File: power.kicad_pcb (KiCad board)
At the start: 2 copper layers, 19.6 x 14.7 mm, 13 parts, among them J6 Conn_01x02, J7 Conn_01x05, Q2 FDC6420C, U5 SGM2036_UTDFN, U7 SGM40561

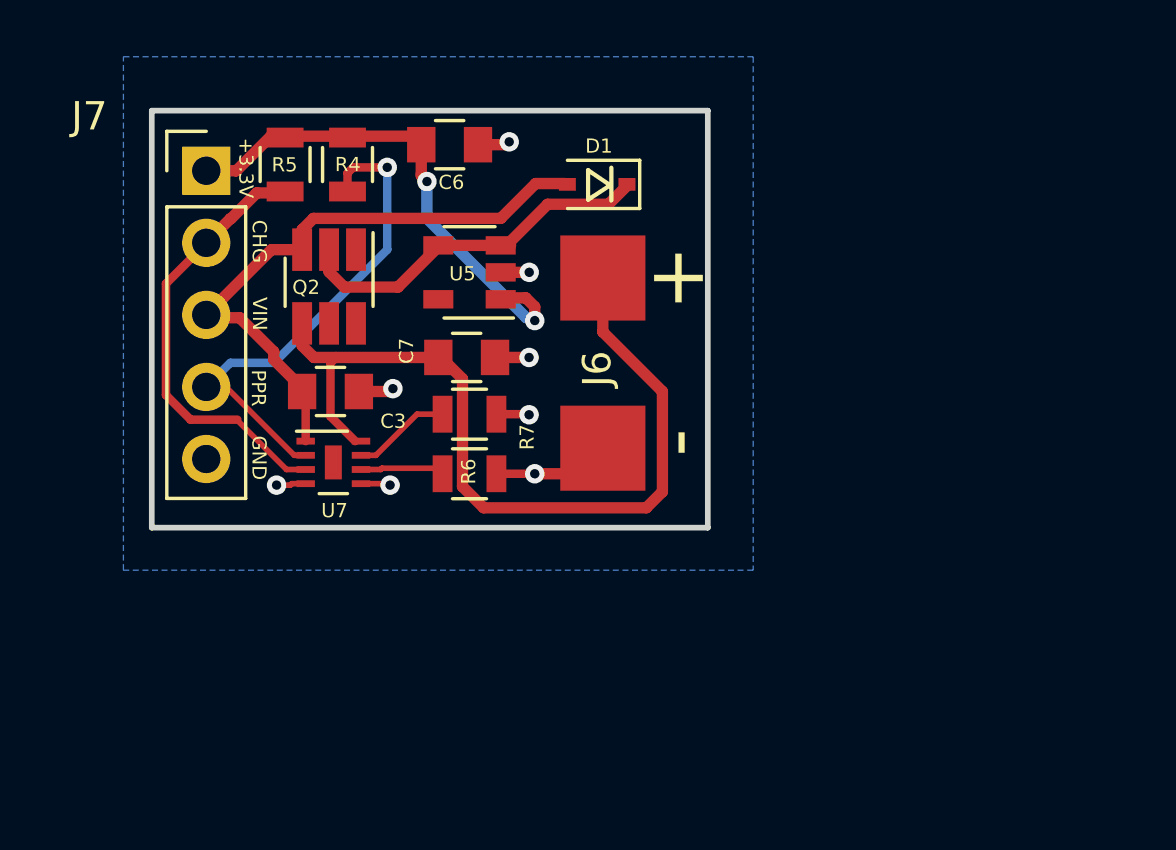
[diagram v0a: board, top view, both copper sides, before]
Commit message: v.01 power board PCB
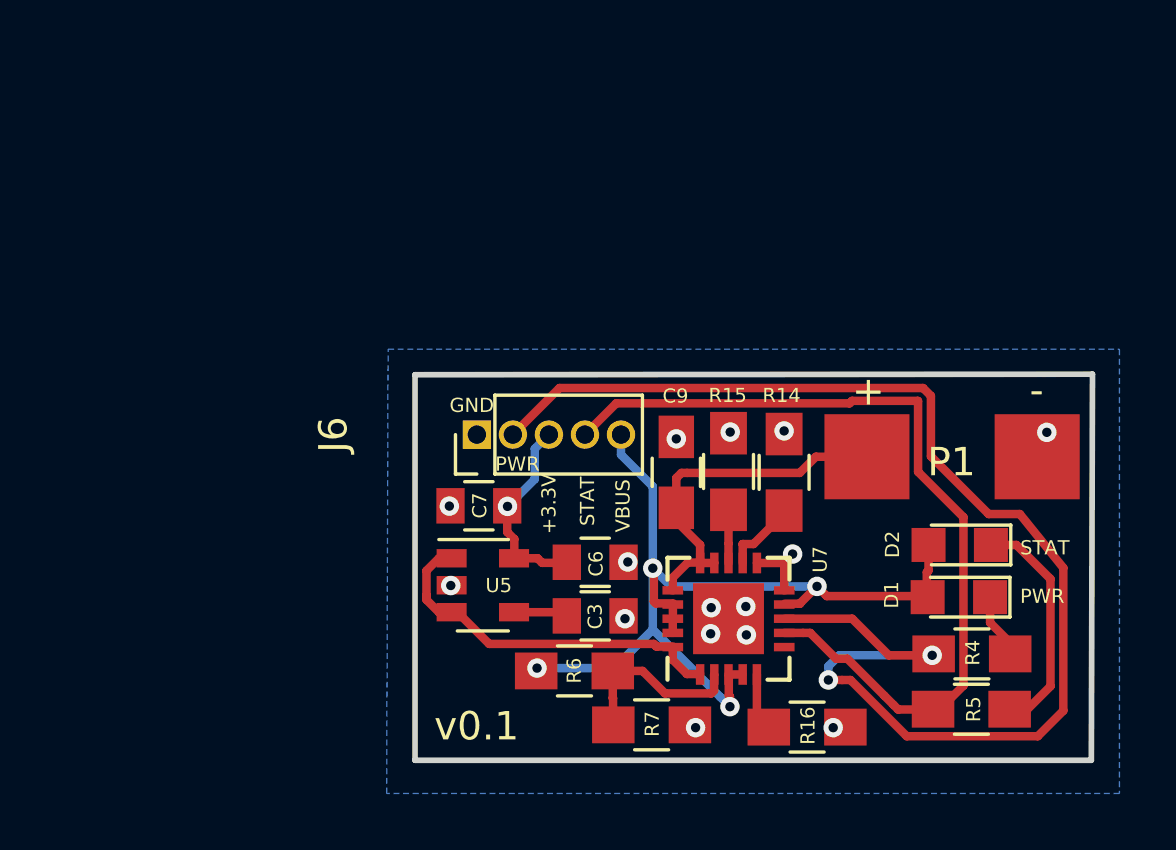
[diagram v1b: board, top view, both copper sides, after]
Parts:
- removed J7: Conn_01x05, Pin_Headers:Pin_Header_Straight_1x05_Pitch2.54mm
- removed Q2: FDC6420C, TO_SOT_Packages_SMD:SuperSOT-6
- added C9: 10uF, Capacitors_SMD:C_0805_HandSoldering, F.Cu at (136.6, 103.8)
- added D2: GREEN, LEDs:LED_0805, F.Cu at (146.6, 106.3)
- added P1: BATT, my-fp-library:Battery Pads 3x3, F.Cu at (146.3, 103.2)
- added R14: 100K, Resistors_SMD:R_0805_HandSoldering, F.Cu at (140.4, 103.8)
- added R15: 1K, Resistors_SMD:R_0805_HandSoldering, F.Cu at (138.4, 103.7)
- added R16: 10K, Resistors_SMD:R_0805_HandSoldering, F.Cu at (141.2, 112.7)
- C3, C7: value 1uF -> 470pF
- C6: value 0.1uF -> 470pF
- D1: value ZLLS410 -> ORANGE; footprint Diodes_SMD:D_SOD-323 -> LEDs:LED_0805
- J6: value Conn_01x02 -> CONN_01X05; footprint my-fp-library:Battery Pads 3x3 -> Pin_Headers:Pin_Header_Straight_1x05_Pitch1.27mm
- R4, R5: value 100K -> 1K; footprint Resistors_SMD:R_0805 -> Resistors_SMD:R_0805_HandSoldering
- R6: value 3M -> 270K; footprint Resistors_SMD:R_0805 -> Resistors_SMD:R_0805_HandSoldering
- R7: value 301K -> 100K; footprint Resistors_SMD:R_0805 -> Resistors_SMD:R_0805_HandSoldering
- U5: value SGM2036_UTDFN -> MIC5219-3.3YM5
- U7: value SGM40561 -> MCP73871-xxI_ML; footprint Housings_DFN_QFN:TDFN-2x2-8L -> Housings_DFN_QFN:QFN-20-1EP_4x4mm_Pitch0.5mm
- moved R5 30.9 mm to (147.0, 112.1), turned to 180 degrees
- moved R4 28.0 mm to (147.0, 110.2), turned to 180 degrees
- moved D1 19.3 mm to (146.6, 108.2)
- moved C6 15.6 mm to (133.7, 106.9)
- moved U7 15.0 mm to (138.4, 108.9), turned to 90 degrees
- moved R7 12.7 mm to (135.7, 112.7)
- moved C3 12.2 mm to (133.7, 108.8)
- moved U5 11.0 mm to (129.8, 107.7), turned to 0 degrees
- moved R6 7.87 mm to (133.0, 110.8)
- moved C7 5.25 mm to (129.6, 104.9), turned to 180 degrees
- moved J6 5.11 mm to (129.6, 102.4), turned to 90 degrees
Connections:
- C3 pad 1: VIN -> Net-(C3-Pad1)
- C7 pad 1: Net-(C7-Pad1) -> +3.3V
- D1 pad 1: +5 -> Net-(D1-Pad1)
- D1 pad 2: VIN -> VBUS
- J6 pad 1: Net-(C7-Pad1) -> (GND)
- J6 pad 2: (GND) -> PWR_SENSE
- R4 pad 1: +3.3V -> Net-(D1-Pad1)
- R4 pad 2: PPR -> PWR_SENSE
- R5 pad 1: +3.3V -> Net-(D2-Pad1)
- R5 pad 2: CHG -> STAT
- R6 pad 1: Net-(R6-Pad1) -> VBUS
- R6 pad 2: (GND) -> Net-(R6-Pad2)
- R7 pad 1: Net-(R7-Pad1) -> Net-(R6-Pad2)
- U5 pad 1: +3.3V -> +5
- U5 pad 4: +5 -> Net-(C3-Pad1)
- U5 pad 5: (no net) -> +3.3V
- U7 pad 1: VIN -> +5
- U7 pad 2: PPR -> Net-(R6-Pad2)
- U7 pad 3: CHG -> VBUS
- U7 pad 4: (GND) -> VBUS
- U7 pad 5: (GND) -> Net-(R16-Pad1)
- U7 pad 6: Net-(R6-Pad1) -> (no net)
- U7 pad 7: Net-(R7-Pad1) -> STAT
- U7 pad 8: Net-(C7-Pad1) -> PWR_SENSE
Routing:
- net PWR_SENSE: track 0.00 -> 48.6 mm, vias 0 -> 2
- net VBUS: track 0.00 -> 33.8 mm, vias 0 -> 4
- net STAT: track 0.00 -> 30.5 mm
- net Net-(C7-Pad1): track 30.1 -> 0.00 mm
- net VIN: track 21.7 -> 0.00 mm
- net PPR: track 19.2 -> 0.00 mm, vias 1 -> 0
- net CHG: track 15.5 -> 0.00 mm
- net Net-(C9-Pad1): track 0.00 -> 13.8 mm
- net +3.3V: track 18.4 -> 6.93 mm, vias 2 -> 1
- net (GND): track 12.4 -> 2.37 mm, vias 8 -> 11
- net Net-(D2-Pad1): track 0.00 -> 8.18 mm
- net Net-(R6-Pad2): track 0.00 -> 6.39 mm
- net Net-(R7-Pad1): track 3.43 -> 0.00 mm
- net Net-(U7-Pad21): track 0.00 -> 3.37 mm, vias 0 -> 4
- net Net-(R6-Pad1): track 2.92 -> 0.00 mm
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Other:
- board size 19.6 x 14.7 mm -> 23.9 x 13.6 mm
- board text added: "PWR"
- board text added: "STAT"
- board text added: "VBUS"
- board text added: "v0.1"
- board text removed: "CHG"
- board text removed: "PPR"
- board text removed: "VIN"
